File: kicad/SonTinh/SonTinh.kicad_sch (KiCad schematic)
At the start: 18 parts, among them IC1 SHT35-DIS-F2.5kS, IC2 STC31-C-R3, IC3 BMP384, J1 Screw_Terminal_01x02, J2 Screw_Terminal_01x02, J3 Screw_Terminal_01x02, J4 Screw_Terminal_01x03, U2 TCA9517ADGK

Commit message: Little Problems
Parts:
- J1, J2: footprint footprints:MKDSFW_15_2_35 -> TerminalBlock_Phoenix:TerminalBlock_Phoenix_PT-1,5-2-3.5-H_1x02_P3.50mm_Horizontal
- J3: footprint footprints:MKDS_15_2_35 -> TerminalBlock_Phoenix:TerminalBlock_Phoenix_PT-1,5-2-3.5-H_1x02_P3.50mm_Horizontal
- J4: footprint footprints:MKDS_15_3_35 -> TerminalBlock_Phoenix:TerminalBlock_Phoenix_PT-1,5-3-3.5-H_1x03_P3.50mm_Horizontal
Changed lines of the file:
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@@
 			)
 		)
-		(property "Footprint" "footprints:MKDSFW_15_2_35"
+		(property "Footprint" "TerminalBlock_Phoenix:TerminalBlock_Phoenix_PT-1,5-2-3.5-H_1x02_P3.50mm_Horizontal"
 			(at 46.99 119.38 0)
 			(effects
@@
 			)
 		)
-		(property "Footprint" "footprints:MKDS_15_2_35"
+		(property "Footprint" "TerminalBlock_Phoenix:TerminalBlock_Phoenix_PT-1,5-2-3.5-H_1x02_P3.50mm_Horizontal"
 			(at 46.99 151.13 0)
 			(effects
@@
 			)
 		)
-		(property "Footprint" "footprints:MKDS_15_3_35"
+		(property "Footprint" "TerminalBlock_Phoenix:TerminalBlock_Phoenix_PT-1,5-3-3.5-H_1x03_P3.50mm_Horizontal"
 			(at 99.06 142.24 0)
 			(effects
@@
 			)
 		)
-		(property "Footprint" "footprints:MKDSFW_15_2_35"
+		(property "Footprint" "TerminalBlock_Phoenix:TerminalBlock_Phoenix_PT-1,5-2-3.5-H_1x02_P3.50mm_Horizontal"
 			(at 46.99 129.54 0)
 			(effects

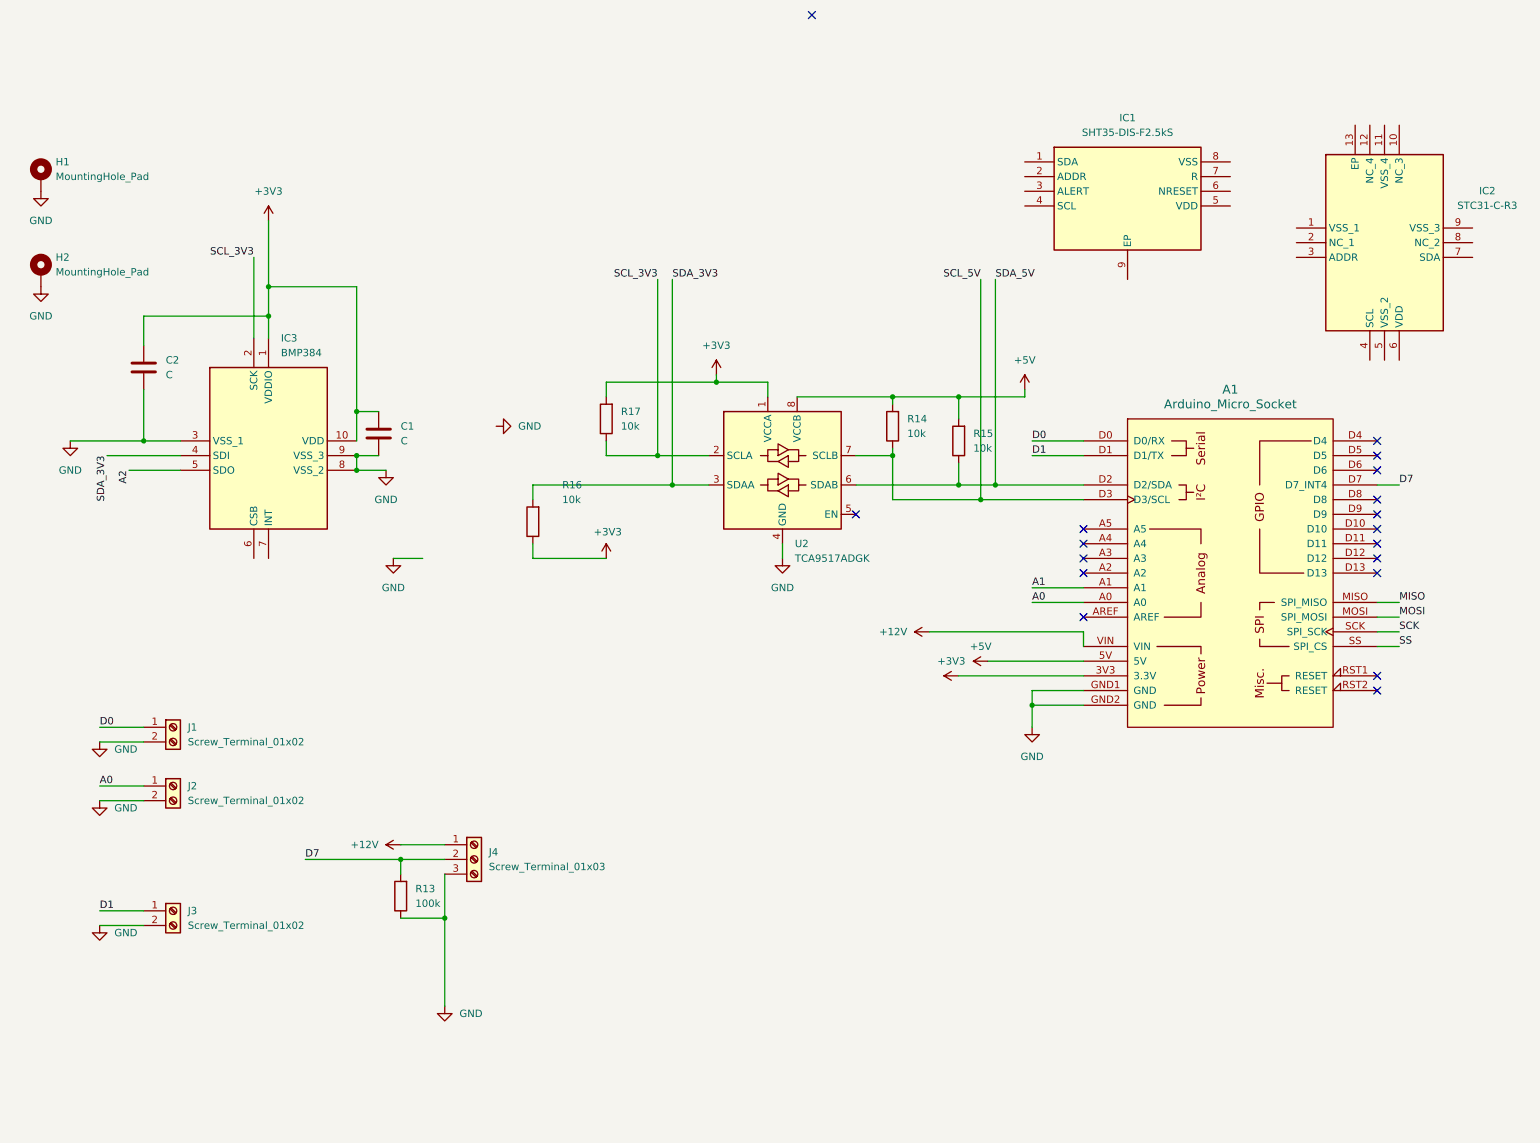
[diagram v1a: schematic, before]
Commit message: Gabrielle's Hope
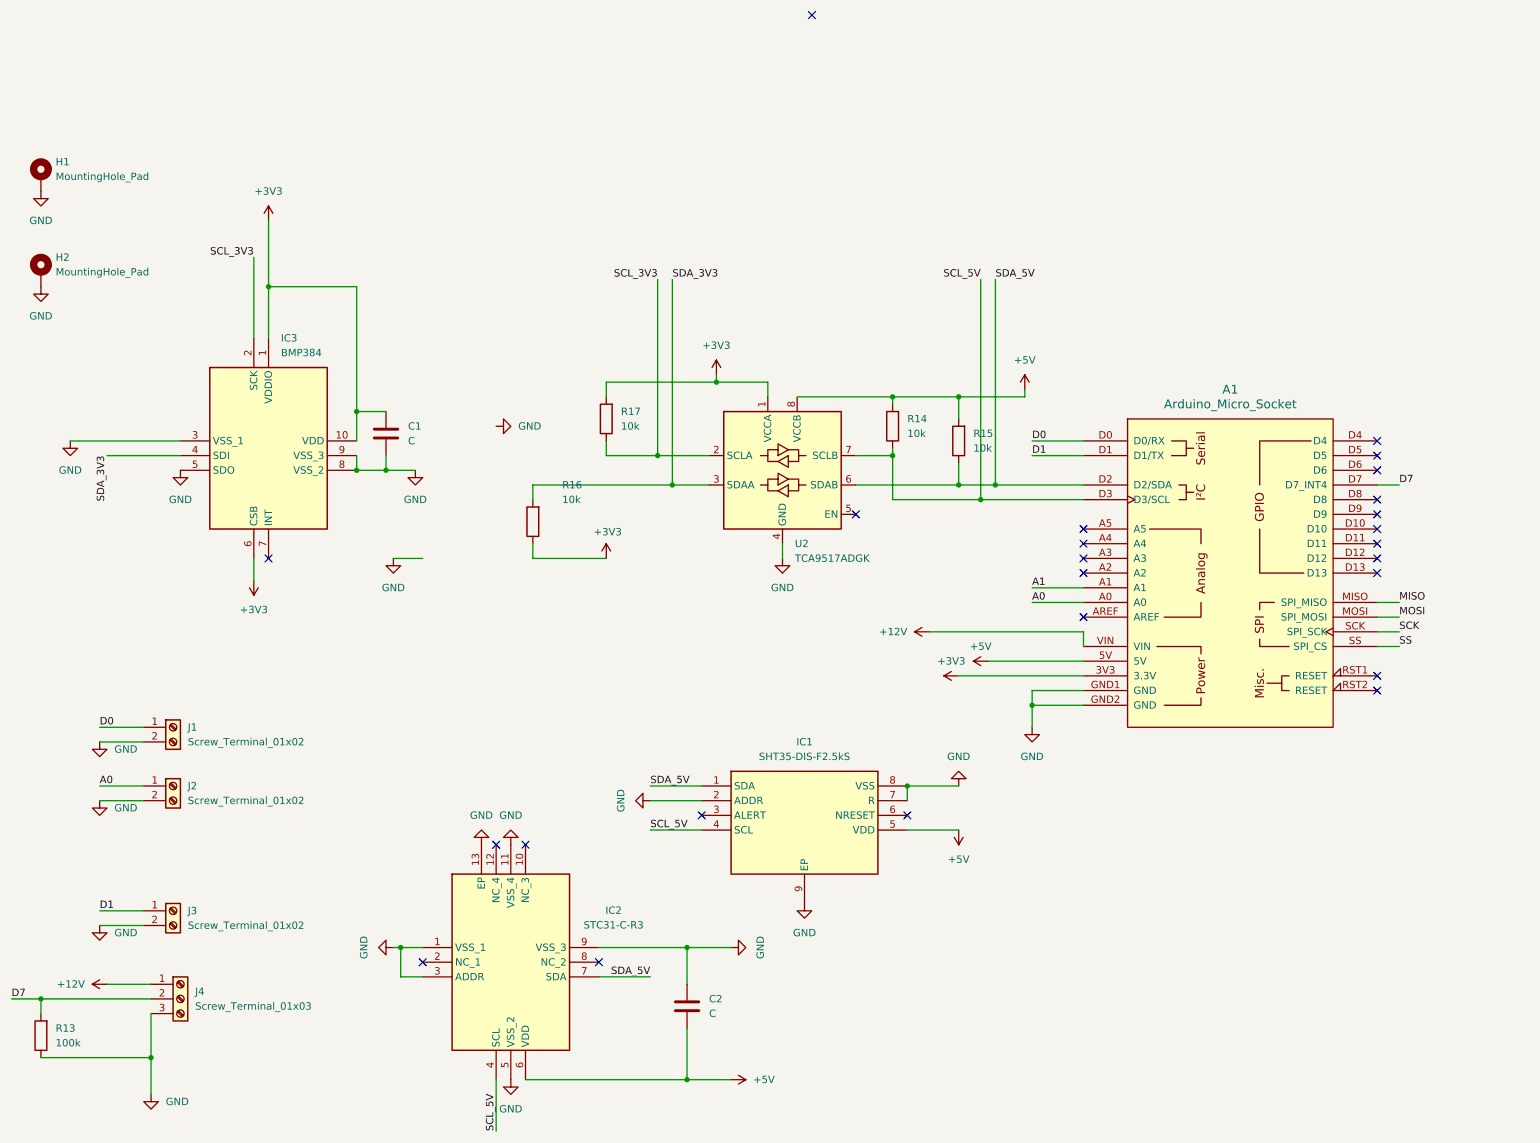
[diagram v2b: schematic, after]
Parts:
- C2: footprint (none) -> Capacitor_SMD:C_0805_2012Metric
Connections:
- net A2 is gone; now on net GND: IC3.5 (SDO)
- net +3V3: now also IC3.6 (CSB); no longer C2.1
- net +5V: now also C2.2, IC1.5 (VDD), IC2.6 (VDD)
- net GND: now also C2.1, IC1.2 (ADDR), IC1.7 (R), IC1.8 (VSS), IC1.9 (EP), IC2.1 (VSS_1), IC2.11 (VSS_4), IC2.13 (EP), IC2.3 (ADDR), IC2.5 (VSS_2), IC2.9 (VSS_3); no longer C2.2
- net SCL_5V: now also IC1.4 (SCL), IC2.4 (SCL)
- net SDA_5V: now also IC1.1 (SDA), IC2.7 (SDA)
- no-connect marks 18 -> 25
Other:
- moved on the sheet: C1, C2, IC1, IC2, J4, R13
